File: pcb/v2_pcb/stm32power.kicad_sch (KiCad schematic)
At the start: 62 parts, among them U2 STM32N657X0H3Q

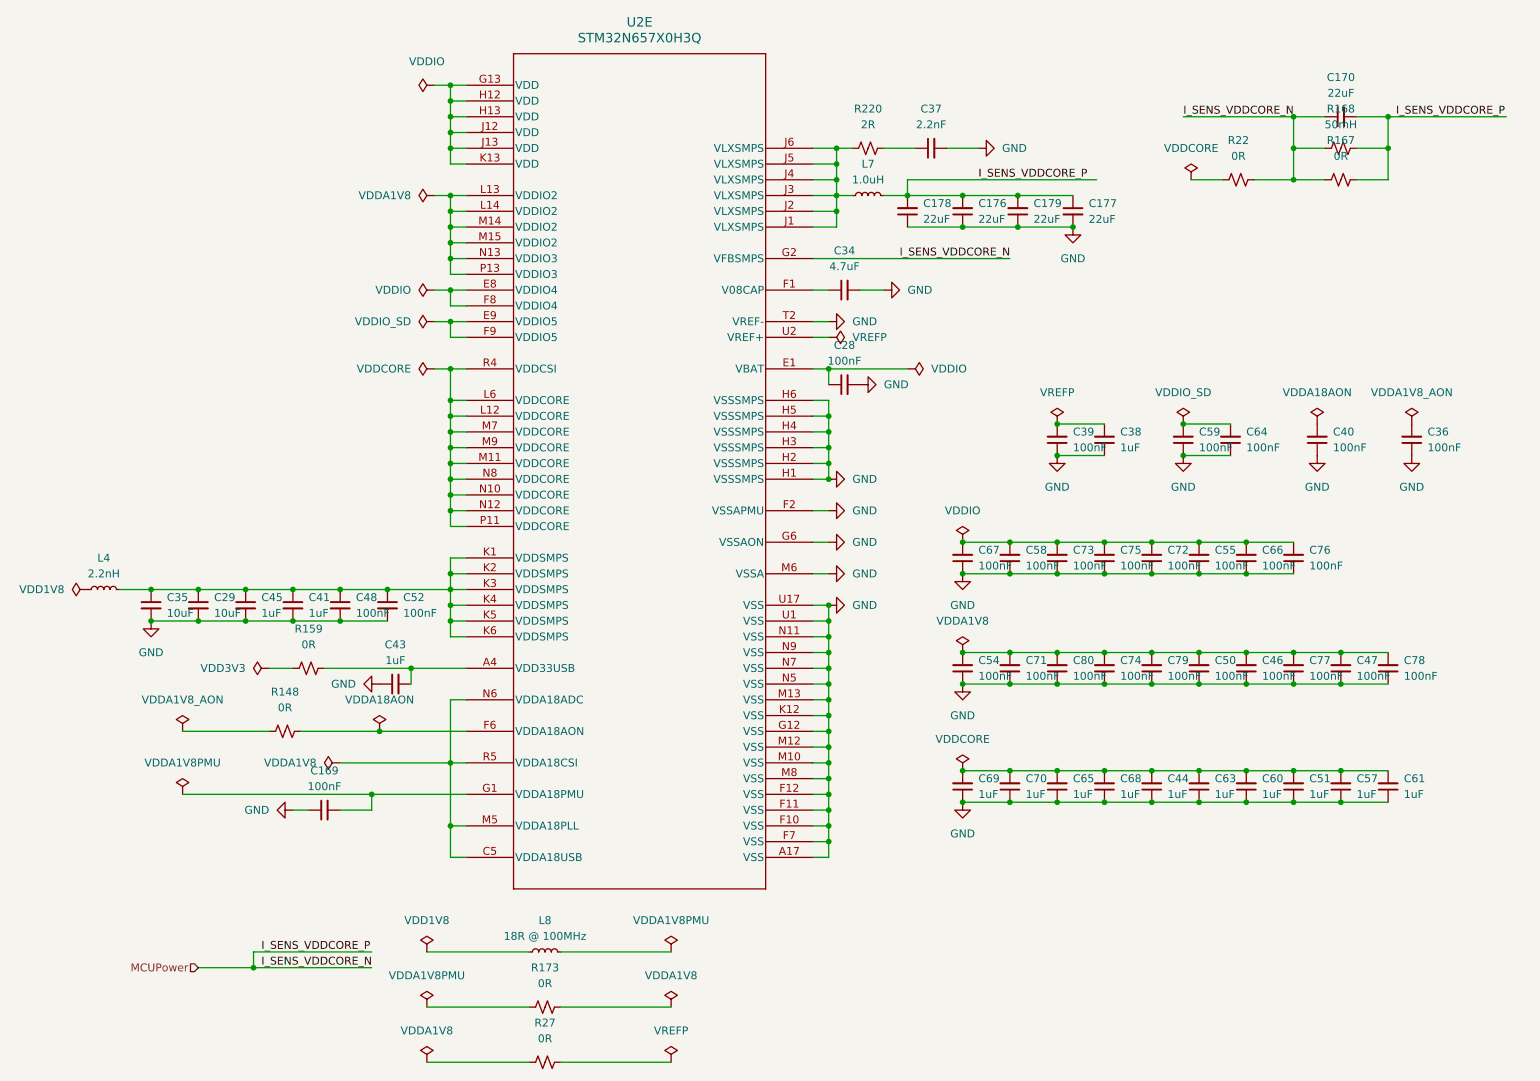
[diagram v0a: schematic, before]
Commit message: add ram
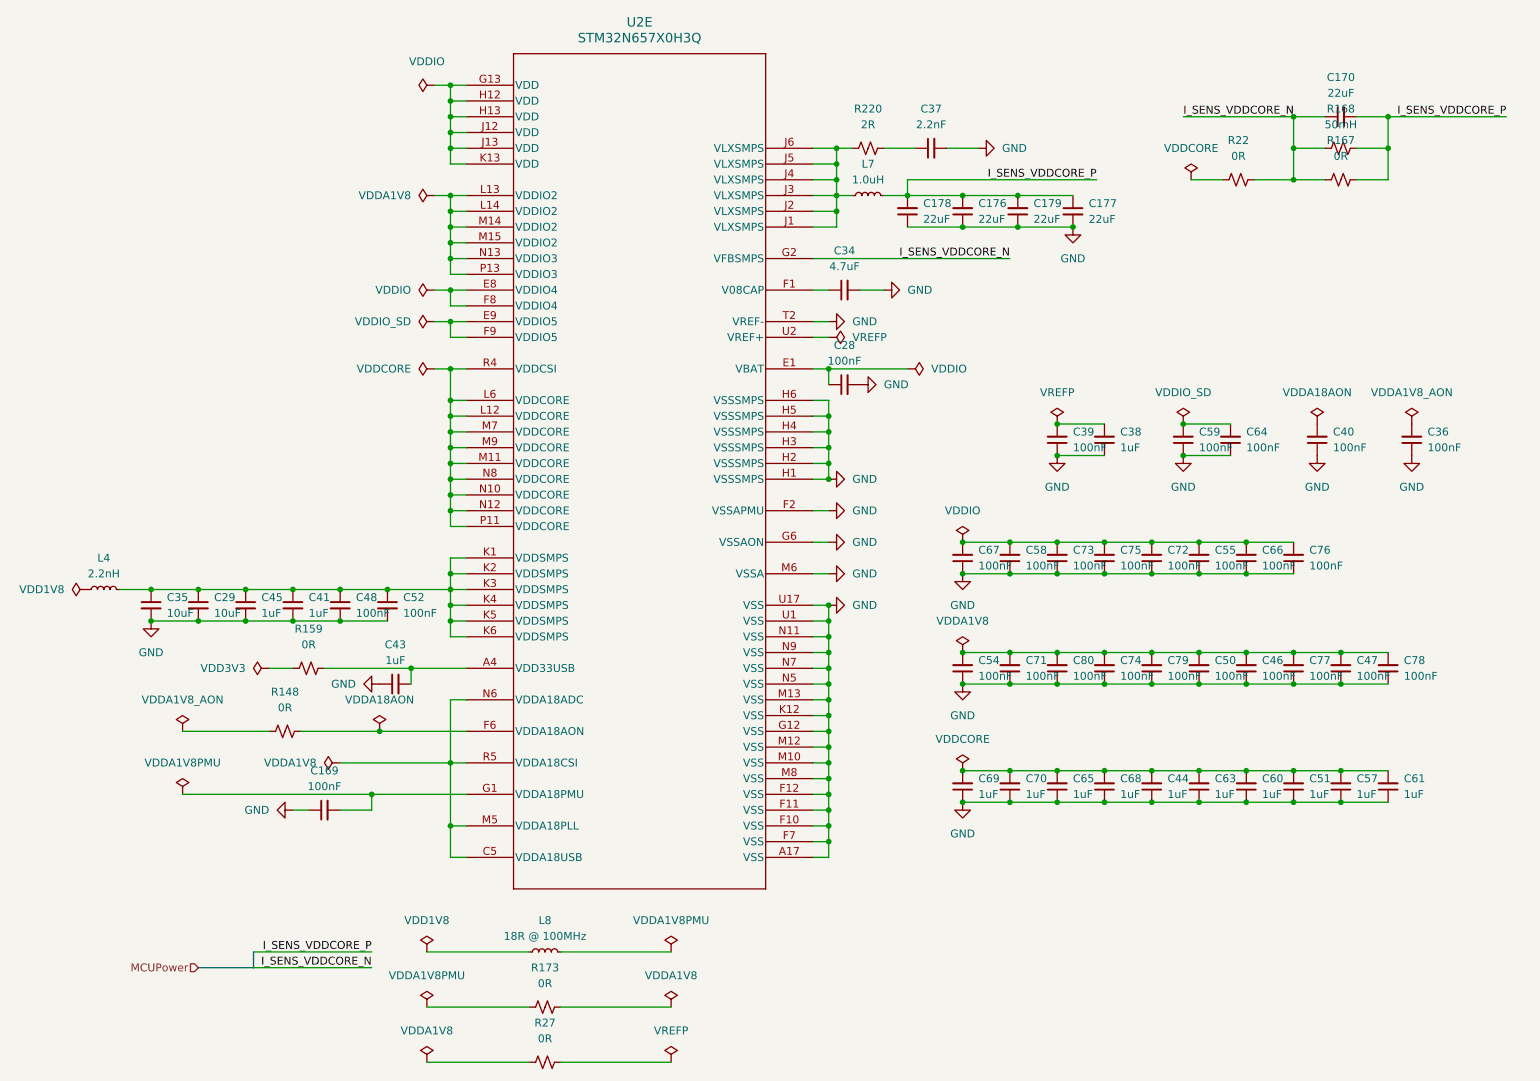
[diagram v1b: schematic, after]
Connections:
- net MCUPower: no longer C170.1, C170.2, C176.2, C177.1, C178.2, C179.2, L7.2, R167.1, R167.2, R168.1, R168.2, R22.2, U2.G2 (VFBSMPS)
- new net I_SENS_VDDCORE_N: C170.1, R167.1, R168.1, R22.2, U2.G2 (VFBSMPS)
- new net I_SENS_VDDCORE_P: C170.2, C176.2, C177.1, C178.2, C179.2, L7.2, R167.2, R168.2
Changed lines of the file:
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@@
-	)
-	(junction
-		(at 50.8 171.45)
-		(diameter 0)
-		(color 0 0 0 0)
 	)
 	(junction
@@
 		)
 	)
+	(bus
+		(pts
+			(xy 41.91 171.45) (xy 50.8 171.45)
+		)
+		(stroke
+			(width 0)
+			(type default)
+		)
+	)
 	(wire
 		(pts
@@
 	(wire
 		(pts
-			(xy 41.91 171.45) (xy 50.8 171.45)
-		)
-		(stroke
-			(width 0)
-			(type default)
-		)
-	)
-	(wire
-		(pts
 			(xy 140.97 133.35) (xy 143.51 133.35)
 		)
@@
 	(wire
 		(pts
+			(xy 50.8 171.45) (xy 69.85 171.45)
+		)
+		(stroke
+			(width 0)
+			(type default)
+		)
+	)
+	(wire
+		(pts
 			(xy 82.55 41.91) (xy 85.09 41.91)
 		)
@@
 		)
 	)
+	(bus
+		(pts
+			(xy 50.8 168.91) (xy 50.8 171.45)
+		)
+		(stroke
+			(width 0)
+			(type default)
+		)
+	)
 	(wire
 		(pts
@@
 	(wire
 		(pts
-			(xy 50.8 168.91) (xy 50.8 171.45)
-		)
-		(stroke
-			(width 0)
-			(type default)
-		)
-	)
-	(wire
-		(pts
 			(xy 140.97 146.05) (xy 143.51 146.05)
 		)
@@
 	(wire
 		(pts
-			(xy 50.8 171.45) (xy 69.85 171.45)
-		)
-		(stroke
-			(width 0)
-			(type default)
-		)
-	)
-	(wire
-		(pts
 			(xy 82.55 82.55) (xy 85.09 82.55)
 		)
@@
 	)
 	(label "I_SENS_VDDCORE_P"
-		(at 234.95 34.29 0)
+		(at 252.73 34.29 180)
 		(effects
 			(font
 				(size 1.27 1.27)
 			)
-			(justify left bottom)
+			(justify right bottom)
 		)
 	)
 	(label "I_SENS_VDDCORE_N"
-		(at 154.94 57.15 0)
+		(at 172.72 57.15 180)
 		(effects
 			(font
 				(size 1.27 1.27)
 			)
-			(justify left bottom)
+			(justify right bottom)
 		)
 	)
 	(label "I_SENS_VDDCORE_P"
-		(at 52.07 168.91 0)
+		(at 69.85 168.91 180)
 		(effects
 			(font
 				(size 1.27 1.27)
 			)
-			(justify left bottom)
+			(justify right bottom)
 		)
 	)
 	(label "I_SENS_VDDCORE_N"
-		(at 52.07 171.45 0)
+		(at 69.85 171.45 180)
 		(effects
 			(font
 				(size 1.27 1.27)
 			)
-			(justify left bottom)
+			(justify right bottom)
 		)
 	)
 	(label "I_SENS_VDDCORE_P"
-		(at 167.64 44.45 0)
+		(at 186.69 44.45 180)
 		(effects
 			(font
 				(size 1.27 1.27)
 			)
-			(justify left bottom)
-		)
-	)
+			(justify right bottom)
+		)
+	)
